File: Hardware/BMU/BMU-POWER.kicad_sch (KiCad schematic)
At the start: 20 parts, among them Q2 AO3401A, U1 TPS54202DDC, U2 TLV75533PDBV

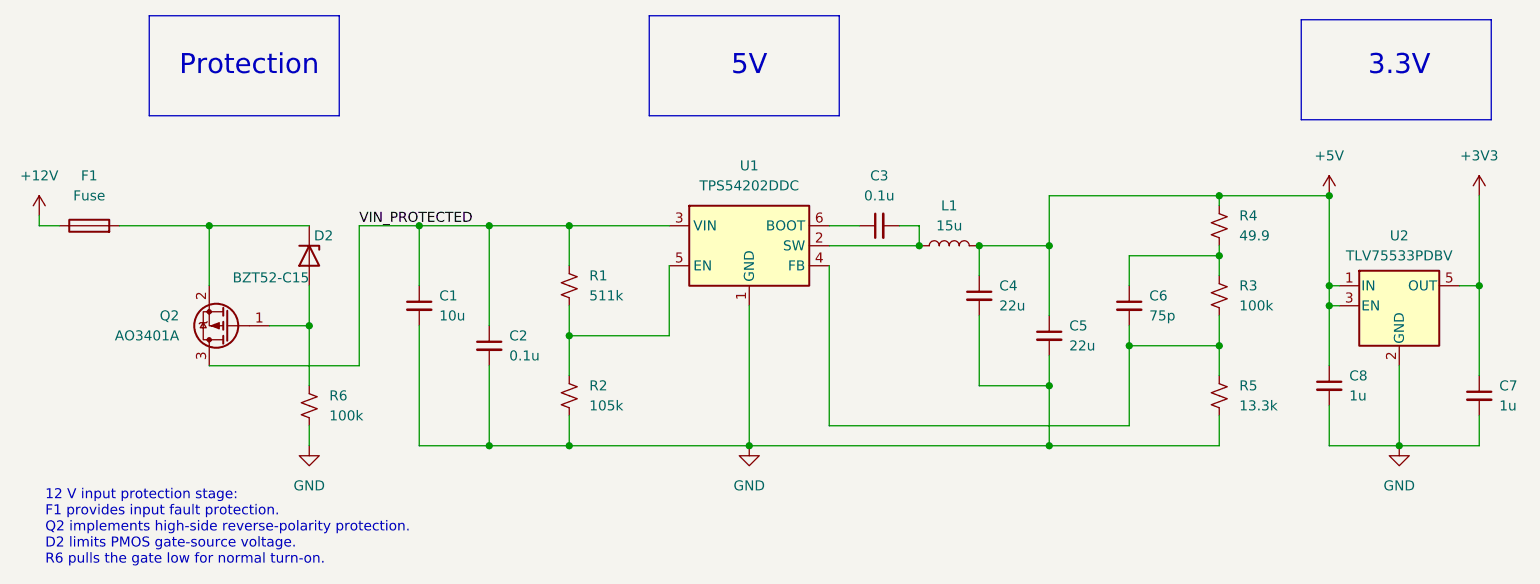
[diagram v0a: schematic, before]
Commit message: update power part
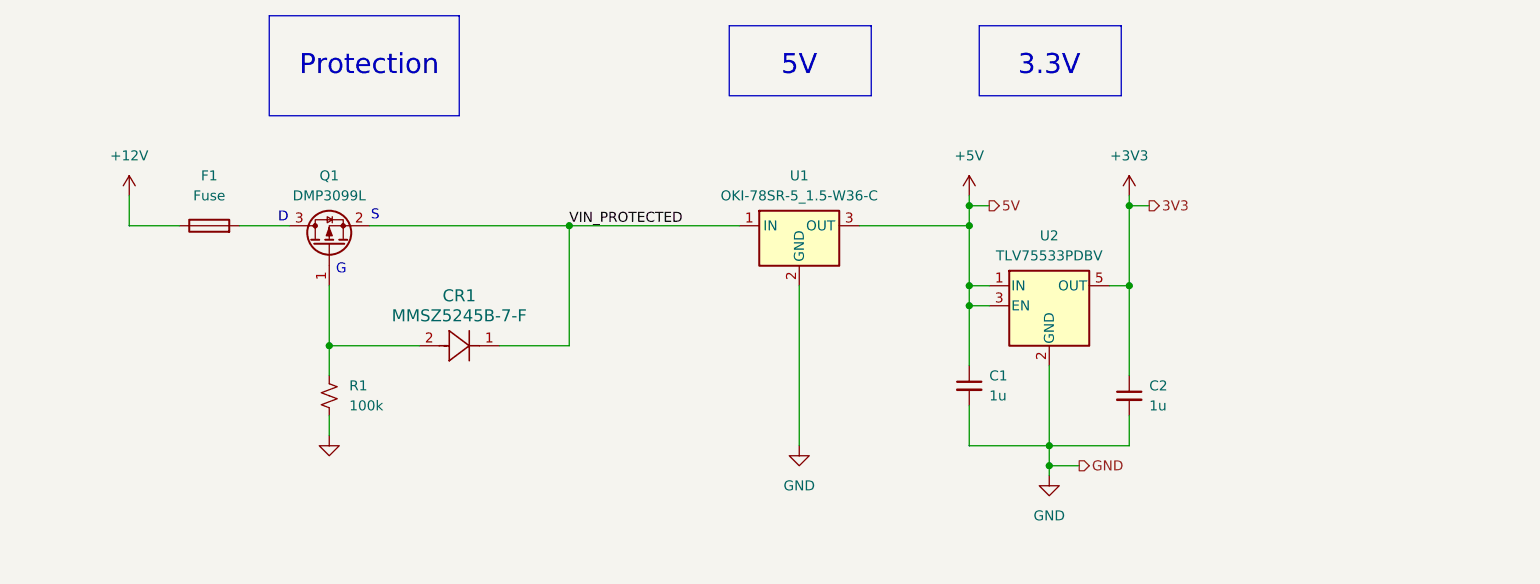
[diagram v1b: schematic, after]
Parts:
- removed C1: 10u, Capacitor_SMD:C_1206_3216Metric, symbol Device:C_Small
- removed C2, C3: 0.1u, Capacitor_SMD:C_0805_2012Metric, symbol Device:C_Small
- removed C4, C5: 22u, Capacitor_SMD:C_1206_3216Metric, symbol Device:C_Small
- removed C6: 75p, Capacitor_SMD:C_0805_2012Metric, symbol Device:C_Small
- removed D2: BZT52-C15, Diode_SMD:D_SOD-123, symbol Device:D_Zener
- removed L1: 15u, Inductor_SMD:L_7.3x7.3_H4.5, symbol Device:L
- removed Q2: AO3401A, Package_TO_SOT_SMD:SOT-23, symbol Transistor_FET:AO3401A
- removed R1: 511k, Resistor_SMD:R_0805_2012Metric, symbol Device:R_Small_US
- removed R2: 105k, Resistor_SMD:R_0805_2012Metric, symbol Device:R_Small_US
- removed R3: 100k, Resistor_SMD:R_0805_2012Metric, symbol Device:R_Small_US
- removed R4: 49.9, Resistor_SMD:R_0805_2012Metric, symbol Device:R_Small_US
- removed R5: 13.3k, Resistor_SMD:R_0805_2012Metric, symbol Device:R_Small_US
- removed U1: TPS54202DDC, Package_TO_SOT_SMD:SOT-23-6, symbol Regulator_Switching:TPS54202DDC
- added CR1: MMSZ5245B-7-F, MMSZ5245B-7-F:SOD123_DIO, symbol 2026-04-30_03-58-02:MMSZ5245B-7-F
- added Q1: DMP3099L, Package_TO_SOT_SMD:SOT-23, symbol Transistor_FET:DMP3099L
- added U1: OKI-78SR-5_1.5-W36-C, Converter_DCDC:Converter_DCDC_Murata_OKI-78SR_Vertical, symbol Converter_DCDC:OKI-78SR-5_1.5-W36-C
- renumbered C8 to C1, C7 to C2, R6 to R1
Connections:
- net +5V: now also U1.3 (OUT)
- net GND: now also U1.2 (GND)
- net VIN_PROTECTED: now also CR1.1, Q1.2 (S), U1.1 (IN)
- net at F1.2: now also Q1.3 (D)
- net at R1.1: now also CR1.2, Q1.1 (G)
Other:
- note added: "D"
- note added: "G"
- note added: "S"
- note removed: "12 V input protection stage: F1 provides input fault protection. Q2 implements high-side reverse-polarity protection. D2 limits PMOS gate-source voltage. R6 pulls the gate low for normal turn-on."
- moved on the sheet: C1, C2, F1, R1, U2
